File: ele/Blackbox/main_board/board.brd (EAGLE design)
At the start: 112.7 x 112.7 mm, 185 parts, among them IC1 DS3231/SO, IC2 QMC5883L-TR, Q2 BSO201SP, Q4 BSS84, Q8 BSO201SP, Q9 BSO201SP, U1 MPU-6050

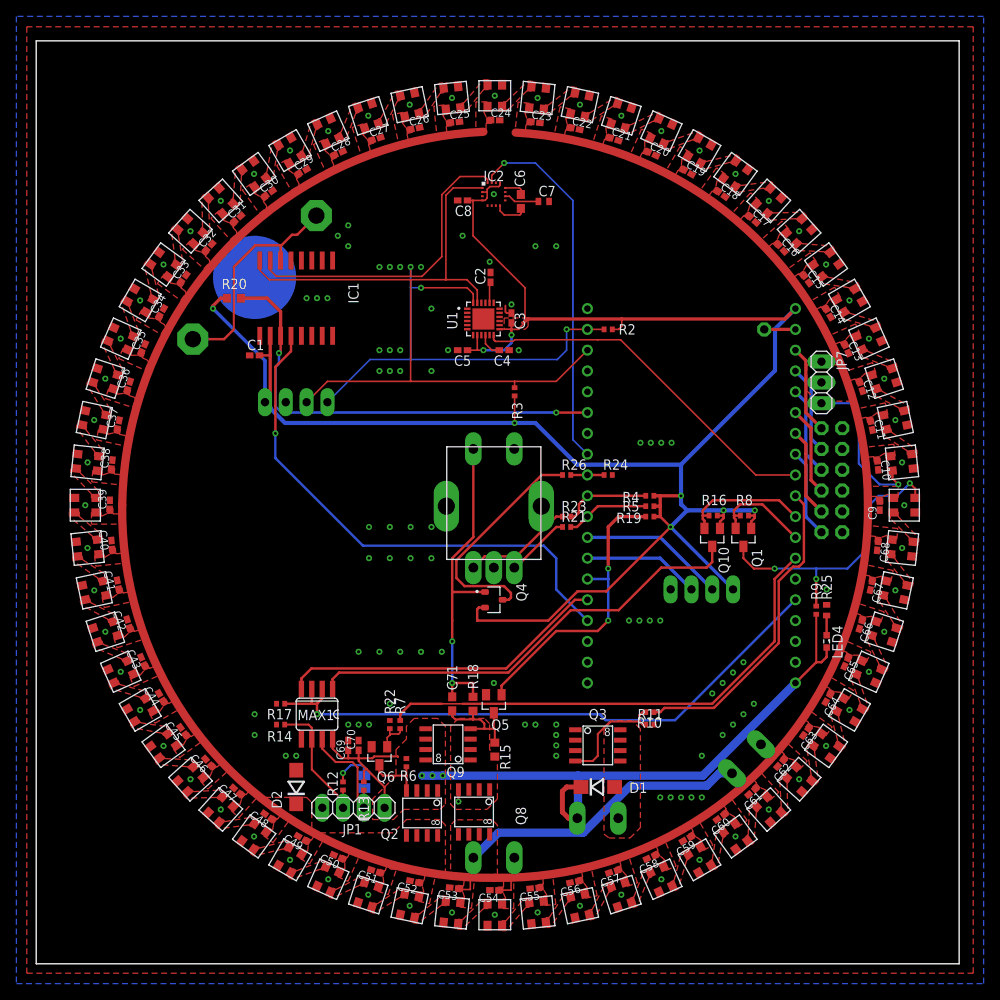
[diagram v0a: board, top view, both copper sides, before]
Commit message: ladeni_drah
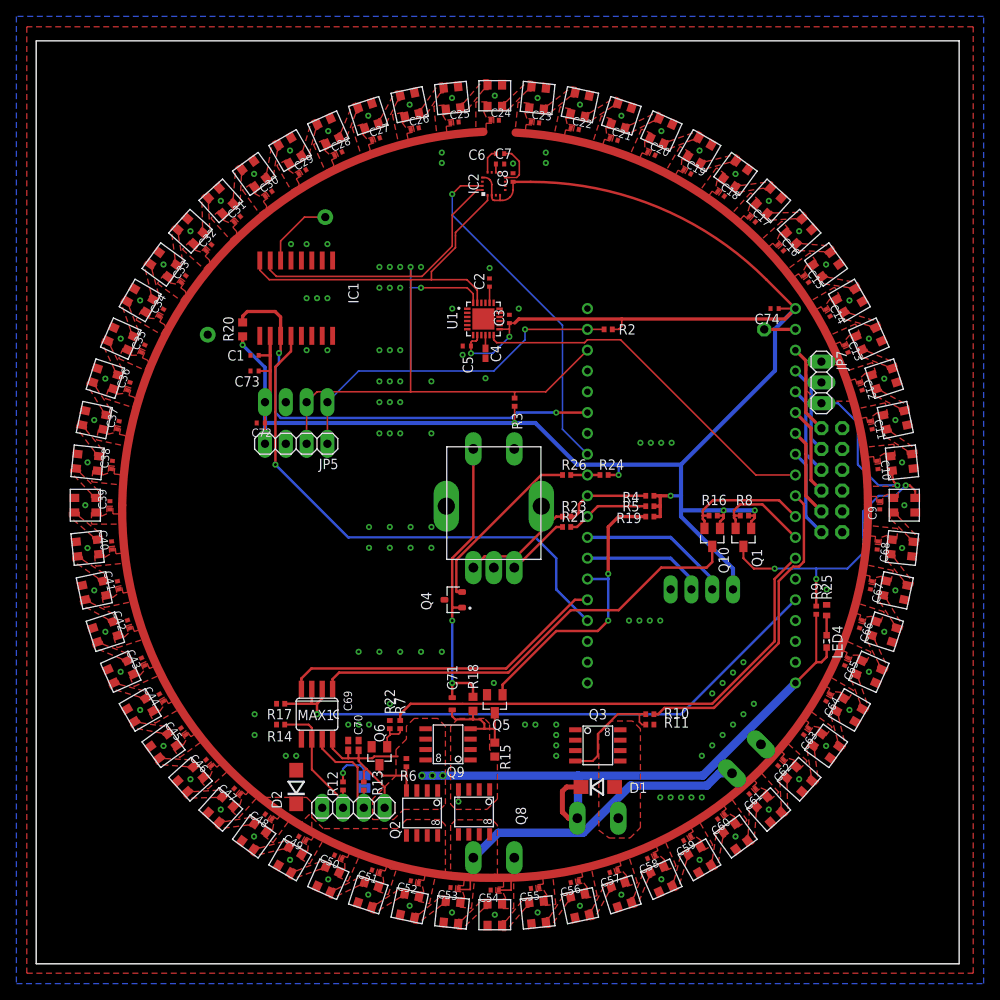
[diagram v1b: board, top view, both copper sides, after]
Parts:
- added C72, C73, C74: 10uf, rcl_upravena:C0402
- added JP5: (no value), pinhead:1X04
- C1, C10, C11, C12, C13, C14, C15, C16, C17, C18, C19, C2, C20, C21, C22, C23, C24, C25, C26, C27, C28, C29, C3, C30, C31, C32, C33, C34, C35, C36, C37, C38, C39, C40, C42, C43, C44, C45, C46, C47, C48, C49, C5, C50, C51, C52, C53, C54, C55, C56, C57, C58, C59, C60, C61, C62, C63, C64, C65, C66, C67, C68, C9: device rcl:C0402K -> rcl_upravena:C0402
- C41: value (none) -> 100pf; device rcl:C0402K -> rcl_upravena:C0402
- C6: device rcl:C0603 -> rcl_upravena:C0402
- C7: device rcl:C0402 -> rcl_upravena:C0402
- C71: device rcl:C0603 -> rcl_upravena:C0603
- C8: device rcl:C0402K -> rcl_upravena:C0402P
- R18: value 2M -> 1M
- R24: value 10k -> 47k
- U$1: value CR2032THM -> CR2032; device CR2032:CR2032-THRU -> CR2032:CH075
- moved C7 7.03 mm to (56.6, 97.7)
- moved C8 6.76 mm to (58.2, 96.0), turned to 90 degrees
- moved C6 6.37 mm to (56.6, 98.9), turned to 0 degrees
- moved Q4 4.95 mm to (50.9, 44.5), turned to 90 degrees
- moved R20 3.96 mm to (25.2, 77.5), turned to 270 degrees
- moved U$1 2.84 mm to (25.4, 81.3)
- moved C4 2.32 mm to (54.9, 74.5), turned to 270 degrees
- moved IC2 1.27 mm to (55.9, 95.2), turned to 90 degrees
- moved R3 1.27 mm to (58.4, 68.6)
- moved C5 0.73 mm to (52.6, 75.4)
- moved C2 0.65 mm to (55.4, 83.2)
- moved R24 0.51 mm to (69.3, 59.7)
- moved C3 0.27 mm to (57.8, 78.7)
- moved R10 0.25 mm to (74.9, 30.5)
- moved Q5 0.12 mm to (56.0, 31.8)
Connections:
- net IO10_NC3 renamed IO9_NC6
- removed net IO11_NC2: IC2.6
- removed net SW!0: Q4.3, R26.1
- new net IO9_NC7: IC2.7
- new net N$7: Q4.2, R26.1
- net +3V3: now also C72.1, C73.1, C74.1, JP5.4, R24.2; no longer Q4.2
- net 3,3!KNOFLIK: now also U$1.+; no longer U$1.+1, U$1.+2
- net GND: now also C72.2, C73.2, C74.2, JP5.3, Q4.3; no longer R24.2
- net IO10_NC2: now also IC2.6; no longer IC2.5
- net IO9_NC2: now also IC2.5; no longer IC2.14
- net IO9_NC3: now also IC2.14; no longer IC2.7
- net SCL: now also JP5.2
- net SDA: now also JP5.1
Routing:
- net SW!0: track 28.6 -> 0.00 mm
- net N$7: track 0.00 -> 21.8 mm
- net 3,3!KNOFLIK: track 27.7 -> 9.05 mm
- net +3V3: track 256.5 -> 251.1 mm
- net SCL: track 95.5 -> 99.9 mm
- net N$66: track 4.31 -> 1.02 mm
- net !SW0: track 39.6 -> 36.6 mm
- net QMC5883-INTERRUPT: track 45.0 -> 42.7 mm
- net SDA: track 98.5 -> 100.2 mm
- net N$62: track 4.11 -> 5.74 mm
- net GND: track 3.04 -> 1.47 mm, vias 138 -> 152
- net N$3: track 3.07 -> 1.62 mm
- net N$9: track 19.2 -> 18.4 mm
- net TX-GPS: track 14.3 -> 15.0 mm
- net RX-GPS: track 17.9 -> 18.6 mm
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- removed copper zone on layer 1, net +3V3
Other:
- board text added: "!+5V"
- board text added: "+5V"
- board text added: "+5v"
- board text added: "A"
- board text added: "B"
- board text added: "GND"
- board text added: "RB3203_BLACK-BOX-BOARD_V1"
